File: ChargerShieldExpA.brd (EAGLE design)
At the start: 161.3 x 99.1 mm, 100 parts, among them IC1 LM324N, IC2 TL431, Q1 BD648, Q2 BUZ11, Q3 BUZ171, Q4 IRFZ48Z, T2 BC548, X1 +Vin, X2 Battery, X3 VCC

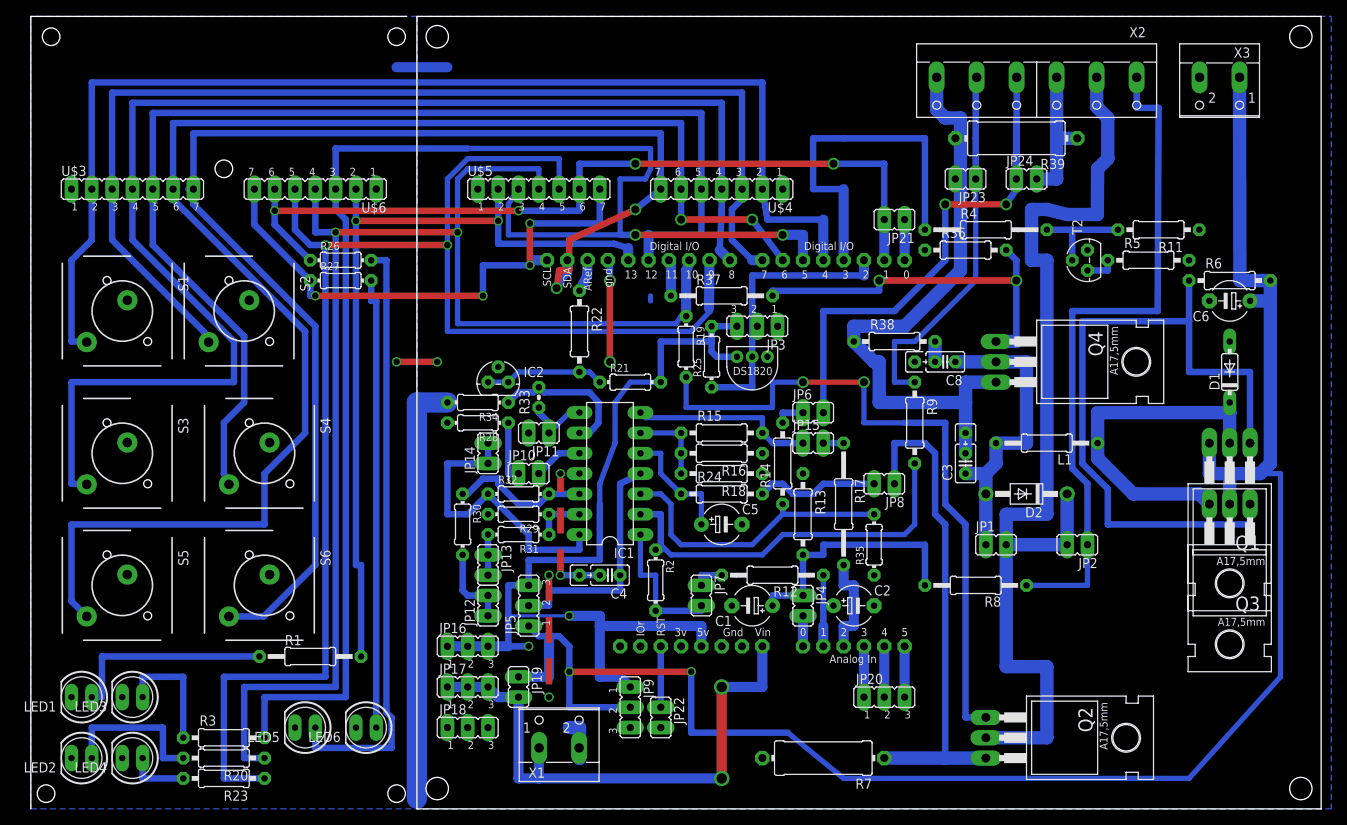
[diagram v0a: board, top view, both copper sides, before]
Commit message: renumbered
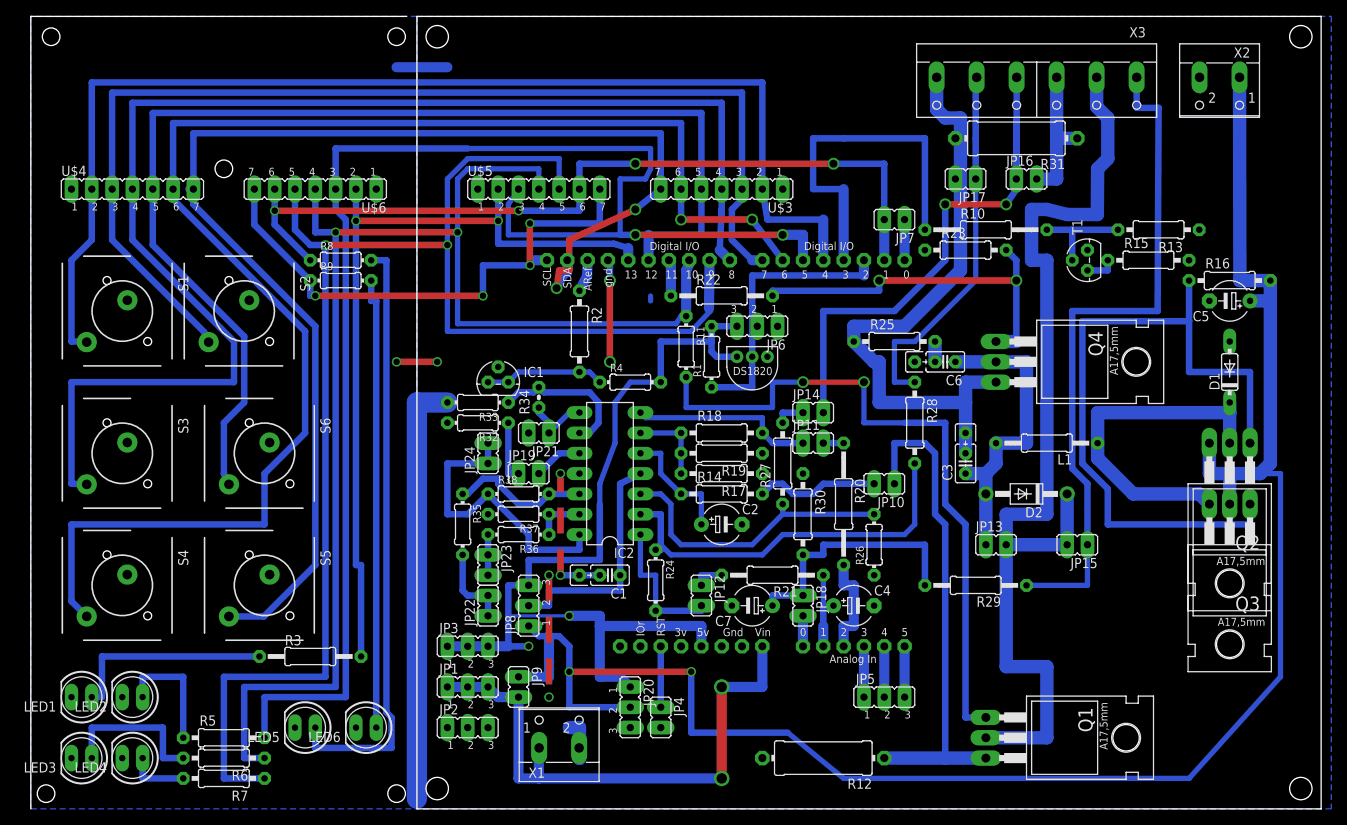
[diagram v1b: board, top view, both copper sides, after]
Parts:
- removed C8: 100n, rcl:C025_050-025X075
- removed R39: 1R666, rcl:0414/15
- added C7: 10µ, rcl:E5-5
- added R10: 2k2, rcl:0207/15
- C1, C6: value 10µ -> 100n; device rcl:E5-5 -> rcl:C025_050-025X075
- C4: value 100n -> 3µ3; device rcl:C025_050-025X075 -> rcl:E5-5
- C5: value 3µ3 -> 10µ
- IC1: value LM324N -> TL431; device linear:DIL14 -> AWJLEagleLib:TO92
- IC2: value TL431 -> LM324N; device AWJLEagleLib:TO92 -> linear:DIL14
- JP1, JP2, JP6, JP8: device bigger:JP1 -> bigger:JP2
- JP16, JP17, JP18, JP9: device bigger:JP2 -> bigger:JP1
- LED2: value (none) -> CHRG2
- LED3: value CHRG2 -> (none)
- Q1: value BD648 -> BUZ11; device transistor-pnp:TO220 -> transistor-fet:TO220
- Q2: value BUZ11 -> BD648; device transistor-fet:TO220 -> transistor-pnp:TO220
- R1: value 470 -> 4k7; device rcl:0207/12 -> rcl:0204/7
- R11: value 100k -> 1k; device rcl:0207/10 -> rcl:0204/7
- R12: value 1k -> 1R666; device rcl:0207/12 -> rcl:0414/15
- R14: value 10k -> 0
- R15: value 100k -> 1k
- R16: value 33k -> 1k
- R17: value 1k -> 12k; device rcl:0207/15 -> rcl:0207/10
- R18: value 12k -> 100k
- R19: value 1k -> 33k; device rcl:0204/7 -> rcl:0207/10
- R2: value 100k -> 4k7; device rcl:0204/7 -> rcl:0207/10
- R20: value 470 -> 1k; device rcl:0207/10 -> rcl:0207/15
- R21: value 200 -> 1k; device rcl:0204/7 -> rcl:0207/12
- R22: value 4k7 -> 200; device rcl:0207/10 -> rcl:0207/12
- R23: value 470 -> 1M
- R24: value 0 -> 100k; device rcl:0207/10 -> rcl:0204/7
- R25: value 4k7 -> 1k; device rcl:0204/7 -> rcl:0207/10
- R26: value 470 -> 100k
- R27: value 470 -> 10k; device rcl:0204/7 -> rcl:0207/10
- R28: value 0 -> 10k; device rcl:0204/7 -> rcl:0207/10
- R29: value 0 -> 1k; device rcl:0204/7 -> rcl:0207/12
- R3: device rcl:0207/10 -> rcl:0207/12
- R30: value 0 -> 100k; device rcl:0204/7 -> rcl:0207/10
- R31: value 0 -> 1R666; device rcl:0204/7 -> rcl:0414/15
- R33: device rcl:0204V -> rcl:0204/7
- R34: device rcl:0204/7 -> rcl:0204V
- R35: value 100k -> 0
- R36: value 1M -> 0; device rcl:0207/10 -> rcl:0204/7
- R37: value 200 -> 0; device rcl:0207/12 -> rcl:0204/7
- R38: value 1k -> 0; device rcl:0207/10 -> rcl:0204/7
- R4: value 2k2 -> 200; device rcl:0207/15 -> rcl:0204/7
- R5, R6: value 1k -> 470
- R7: value 1R666 -> 470; device rcl:0414/15 -> rcl:0207/10
- R8: value 1k -> 470; device rcl:0207/12 -> rcl:0204/7
- R9: value 10k -> 470; device rcl:0207/10 -> rcl:0204/7
- S4: value Discharge -> A
- S5: value A -> B
- S6: value B -> Discharge
- U$1: value ARDUINOR3BPLACE-LONG -> DS1820TO92; device arduino-long:ARDUINOR3-BPLACE-LONG -> Ava:DS1820
- U$2: value DS1820TO92 -> ARDUINOR3BPLACE-LONG; device Ava:DS1820 -> arduino-long:ARDUINOR3-BPLACE-LONG
- X2: value Battery -> VCC; device con-wago-500:W237-6 -> con-wago-500:W237-102
- X3: value VCC -> Battery; device con-wago-500:W237-102 -> con-wago-500:W237-6
- moved R6 139.2 mm to (-21.6, -11.4), turned to 180 degrees
- moved R5 130.1 mm to (-21.6, -8.89)
- moved R23 113.8 mm to (71.1, 52.1), turned to 0 degrees
- moved JP16 91.1 mm to (78.7, 61.0), turned to 270 degrees
- moved R8 89.2 mm to (-6.99, 50.8), turned to 0 degrees
- moved JP17 88.9 mm to (71.1, 61.0), turned to 90 degrees
- moved R20 83.7 mm to (55.9, 20.3), turned to 270 degrees
- moved JP2 79.6 mm to (8.89, -7.62), turned to 0 degrees
- moved R31 79.5 mm to (77.5, 66.0)
- moved JP23 76.8 mm to (11.4, 12.7), turned to 180 degrees
- moved R26 75.6 mm to (59.7, 15.2), turned to 90 degrees
- moved JP24 75.5 mm to (11.4, 26.7), turned to 0 degrees
- moved R7 75.0 mm to (-21.6, -14.0)
- moved R9 73.9 mm to (-6.99, 48.3), turned to 0 degrees
- moved U$3 73.7 mm to (40.6, 59.7), turned to 180 degrees
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- renumbered T2 to T1
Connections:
- net +5V: now also JP20.1, JP3.1, JP3.2, JP6.3, JP8.3, R1.2, R4.2, U$1.VDD, U$2.5V; no longer JP16.1, JP16.2, JP16.3, JP5.3, JP9.1, R21.2, R25.2, U$1.5V, U$2.VDD
- net 3V: now also U$2.3V; no longer U$1.3V
- net GND: now also C1.2, C4.-, C7.-, IC1.2, IC2.11, JP17.2, JP2.1, JP2.2, JP2.3, JP20.3, JP4.2, JP6.1, R12.2, R17.1, R19.1, R23.1, R25.1, R26.1, R30.1, R31.2, R32.2, R33.2, R37.2, U$2.GND1, U$2.GND2, X2.2, X3.6; no longer C1.-, C4.2, C6.-, IC1.11, IC2.2, JP18.1, JP18.2, JP18.3, JP22.2, JP23.2, JP3.1, JP9.3, R11.1, R16.1, R18.1, R28.2, R29.2, R34.2, R35.1, R36.1, R38.1, R39.2, R7.2, U$1.GND1, U$1.GND2, X2.6, X3.2
- net I1_SENSE+: now also JP16.2, R31.1, X3.3; no longer JP24.2, R39.1, X2.3
- net I1_SENSE-: now also JP17.1, R28.1, X3.5; no longer JP23.1, R9.1, X2.5
- net I_BATT1: now also C4.+, R21.1, U$2.A1; no longer C2.+, R12.1, U$1.A1
- net I_BATT2: now also JP5.2, U$2.A4; no longer JP20.2, U$1.A4
- net I_DISC1: now also R20.2, U$2.A2; no longer R17.2, U$1.A2
- net I_DISC2: now also JP5.3, U$2.A5; no longer JP20.3, U$1.A5
- net N$1: now also R3.2, U$2.D13; no longer R1.2, U$1.D13
- net N$10: now also C6.1, JP13.1; no longer C8.1, JP1.1
- net N$11: now also IC2.1, JP12.2, R24.2; no longer IC1.1, JP7.2, R2.2
- net N$12: now also JP6.2, R1.1, U$1.DQ, U$2.D2; no longer JP3.2, R25.1, U$1.D2, U$2.DQ
- net N$13: now also JP13.2, JP15.2, Q1.2, X3.2; no longer JP1.2, JP2.2, Q2.2, X2.2
- net N$14: now also IC2.2, R24.1, R28.2; no longer IC1.2, R2.1, R9.2
- net N$15: now also IC2.3, R26.2, R27.1; no longer IC1.3, R14.1, R35.2
- net N$16: now also IC2.6, R17.2, R18.1, R19.2; no longer IC1.6, R15.1, R16.2, R18.2
- net N$17: now also IC2.7, JP11.1, R18.2; no longer IC1.7, JP15.1, R15.2
- net N$18: now also Q1.1, R11.2; no longer Q2.1, R19.2
- net N$19: now also R5.2, U$2.D5; no longer R3.2, U$1.D5
- net N$2: now also R3.1; no longer R1.1
- net N$20: now also LED3.A, R6.2; no longer LED2.A, R20.2
- net N$21: now also R7.2; no longer R23.2
- net N$22: now also JP14.1, R27.2; no longer JP6.1, R14.2
- net N$23: now also S6.3, U$2.D12; no longer S4.3, U$1.D12
- net N$24: now also LED2.A, R5.1; no longer LED3.A, R3.1
- net N$25: now also JP10.1, Q1.3, R12.1; no longer JP8.1, Q2.3, R7.1
- net N$26: now also U$2.D4; no longer U$1.D4
- net N$27: now also IC1.1, IC1.3, R2.2, R4.1; no longer IC2.1, IC2.3, R21.1, R22.2
- net N$28: now also R2.1, U$2.AREF; no longer R22.1, U$1.AREF
- net N$29: now also C2.+, IC2.5, R14.1; no longer C5.+, IC1.5, R24.1
- net N$3: now also C7.+, JP18.1, R29.2, R30.2; no longer C1.+, JP4.1, R13.2, R8.2
- net N$30: now also U$2.D7; no longer U$1.D7
- net N$31: now also U$2.D8; no longer U$1.D8
- net N$32: now also JP12.1, R21.2; no longer JP7.1, R12.2
- net N$33: now also JP10.2, R14.2; no longer JP8.2, R24.2
- net N$34: now also IC2.8, JP21.1, R34.1; no longer IC1.8, JP11.1, R33.1
- net N$35: now also JP11.2, R20.1; no longer JP15.2, R17.1
- net N$36: now also IC2.13, R36.1, R37.1; no longer IC1.13, R29.1, R31.1
- net N$37: now also S4.3, U$2.D6; no longer S5.3, U$1.D6
- net N$38: now also S5.3, U$2.SDA; no longer S6.3, U$1.SDA
- net N$39: now also R8.2; no longer R26.2
- net N$4: now also C1.1, IC2.4, JP8.2; no longer C4.1, IC1.4, JP5.2
- net N$40: now also R9.2; no longer R27.2
- net N$41: now also R9.1, U$2.SCL; no longer R27.1, U$1.SCL
- net N$42: now also JP7.2, R8.1, U$2.D1; no longer JP21.2, R26.1, U$1.D1
- net N$43: now also IC2.10, JP19.2; no longer IC1.10, JP10.2
- net N$44: now also JP19.1, R32.1; no longer JP10.1, R28.1
- net N$45: now also IC2.12, R35.1, R38.2; no longer IC1.12, R30.1, R32.2
- net N$46: now also JP22.1, JP22.2, R35.2; no longer JP12.1, JP12.2, R30.2
- net N$47: now also JP23.1, JP23.2, R36.2; no longer JP13.1, JP13.2, R31.2
- net N$48: now also IC2.14, JP24.1, JP24.2, R38.1; no longer IC1.14, JP14.1, JP14.2, R32.1
- net N$49: now also IC2.9, R33.1, R34.2; no longer IC1.9, R33.2, R34.1
- net N$5: now also R10.2, R13.2; no longer R11.2, R4.2
- net N$50: now also C6.2, R25.2; no longer C8.2, R38.2
- net N$51: now also R22.2, R23.2; no longer R36.2, R37.2
- net N$52: now also JP7.1, U$2.D0; no longer JP21.1, U$1.D0
- net N$53: now also JP4.1, U$2.RESET; no longer JP22.1, U$1.RESET
- net N$54: now also JP14.2, JP16.1, X3.4; no longer JP24.1, JP6.2, X2.4
- net N$6: now also R15.1; no longer R5.1
- net N$7: now also Q2.1, R15.2, R16.1; no longer Q1.1, R5.2, R6.1
- net N$8: now also JP15.1, R29.1, X3.1; no longer JP2.1, R8.1, X2.1
- net N$9: now also Q2.2; no longer Q1.2
- net PWM_CHARGE1: now also R10.1, U$2.D3; no longer R4.1, U$1.D3
- net PWM_CHARGE2: now also R22.1, U$2.D11; no longer R37.1, U$1.D11
- net PWM_DISCHARGE1: now also R11.1, R6.1, U$2.D10; no longer R19.1, R20.1, U$1.D10
- net PWM_DISCHARGE2: now also R7.1, U$2.D9; no longer R23.1, U$1.D9
- net U_BATT1: now also JP18.2, U$2.A0; no longer JP4.2, U$1.A0
- net U_BATT2: now also JP5.1, U$2.A3; no longer JP20.1, U$1.A3
- net VCC: now also C5.+, JP20.2, JP8.1, JP9.1, Q2.3, R16.2, X2.1; no longer C6.+, JP19.1, JP5.1, JP9.2, Q1.3, R6.2, X3.1
- net VIN: now also JP1.1, JP1.2, JP1.3, JP9.2, U$2.VIN; no longer JP17.1, JP17.2, JP17.3, JP19.2, U$1.VIN
